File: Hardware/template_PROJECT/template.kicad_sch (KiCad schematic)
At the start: 7 parts

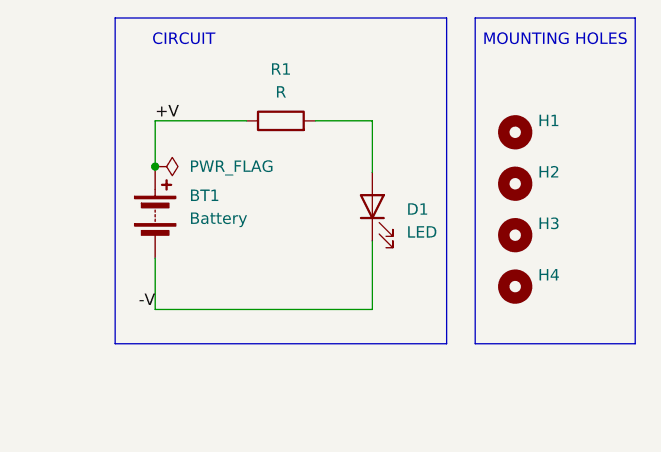
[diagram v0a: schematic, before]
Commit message: creating errors to check
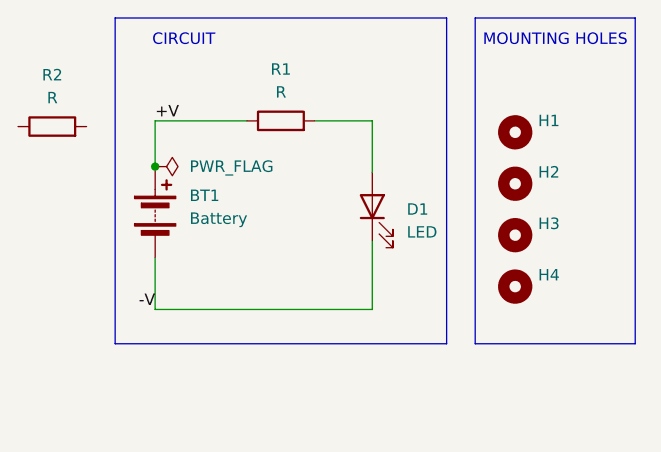
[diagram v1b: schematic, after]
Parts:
- added R2: R, Resistor_SMD:R_0805_2012Metric, symbol Device:R
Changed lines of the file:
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@@
+		)
+	)
+	(symbol
+		(lib_id "Device:R")
+		(at 120.65 92.71 90)
+		(unit 1)
+		(exclude_from_sim no)
+		(in_bom yes)
+		(on_board yes)
+		(dnp no)
+		(fields_autoplaced yes)
+		(property "Reference" "R2"
+			(at 120.65 86.995 90)
+			(effects
+				(font
+					(size 1.27 1.27)
+				)
+			)
+		)
+		(property "Value" "R"
+			(at 120.65 89.535 90)
+			(effects
+				(font
+					(size 1.27 1.27)
+				)
+			)
+		)
+		(property "Footprint" "Resistor_SMD:R_0805_2012Metric"
+			(at 120.65 94.488 90)
+			(effects
+				(font
+					(size 1.27 1.27)
+				)
+				(hide yes)
+			)
+		)
+		(property "Datasheet" "~"
+			(at 120.65 92.71 0)
+			(effects
+				(font
+					(size 1.27 1.27)
+				)
+				(hide yes)
+			)
+		)
+		(property "Description" "Resistor"
+			(at 120.65 92.71 0)
+			(effects
+				(font
+					(size 1.27 1.27)
+				)
+				(hide yes)
+			)
+		)
+		(pin "1"
+		)
+		(pin "2"
+		)
+		(instances
+			(project "template"
+				(path "/92a86815-0425-4ac3-80bb-037195814139"
+					(reference "R2")
+					(unit 1)
+				)
+			)
 		)
 	)

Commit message: worked
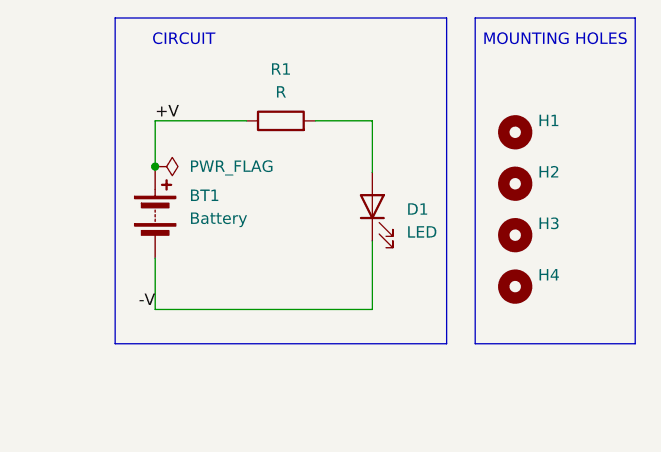
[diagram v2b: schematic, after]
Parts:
- removed R2: R, Resistor_SMD:R_0805_2012Metric, symbol Device:R
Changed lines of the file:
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@@
-		)
-	)
-	(symbol
-		(lib_id "Device:R")
-		(at 120.65 92.71 90)
-		(unit 1)
-		(exclude_from_sim no)
-		(in_bom yes)
-		(on_board yes)
-		(dnp no)
-		(fields_autoplaced yes)
-		(property "Reference" "R2"
-			(at 120.65 86.995 90)
-			(effects
-				(font
-					(size 1.27 1.27)
-				)
-			)
-		)
-		(property "Value" "R"
-			(at 120.65 89.535 90)
-			(effects
-				(font
-					(size 1.27 1.27)
-				)
-			)
-		)
-		(property "Footprint" "Resistor_SMD:R_0805_2012Metric"
-			(at 120.65 94.488 90)
-			(effects
-				(font
-					(size 1.27 1.27)
-				)
-				(hide yes)
-			)
-		)
-		(property "Datasheet" "~"
-			(at 120.65 92.71 0)
-			(effects
-				(font
-					(size 1.27 1.27)
-				)
-				(hide yes)
-			)
-		)
-		(property "Description" "Resistor"
-			(at 120.65 92.71 0)
-			(effects
-				(font
-					(size 1.27 1.27)
-				)
-				(hide yes)
-			)
-		)
-		(pin "1"
-		)
-		(pin "2"
-		)
-		(instances
-			(project "template"
-				(path "/92a86815-0425-4ac3-80bb-037195814139"
-					(reference "R2")
-					(unit 1)
-				)
-			)
 		)
 	)

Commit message: should fail now
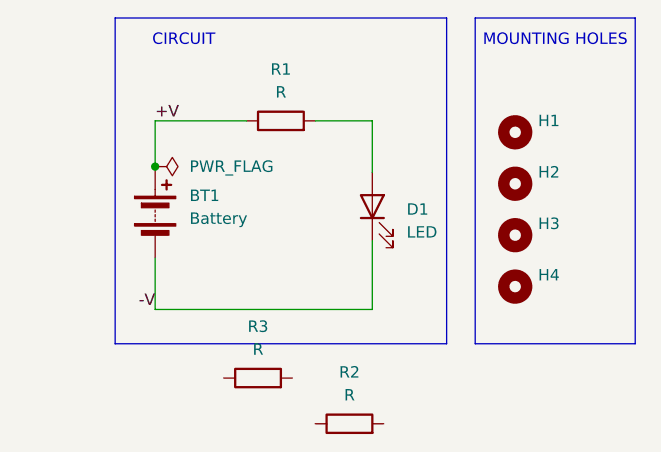
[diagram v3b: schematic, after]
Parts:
- added R2, R3: R, Resistor_SMD:R_0805_2012Metric, symbol Device:R
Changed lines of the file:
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@@
+		)
+	)
+	(symbol
+		(lib_id "Device:R")
+		(at 153.67 125.73 90)
+		(unit 1)
+		(exclude_from_sim no)
+		(in_bom yes)
+		(on_board yes)
+		(dnp no)
+		(fields_autoplaced yes)
+		(property "Reference" "R2"
+			(at 153.67 120.015 90)
+			(effects
+				(font
+					(size 1.27 1.27)
+				)
+			)
+		)
+		(property "Value" "R"
+			(at 153.67 122.555 90)
+			(effects
+				(font
+					(size 1.27 1.27)
+				)
+			)
+		)
+		(property "Footprint" "Resistor_SMD:R_0805_2012Metric"
+			(at 153.67 127.508 90)
+			(effects
+				(font
+					(size 1.27 1.27)
+				)
+				(hide yes)
+			)
+		)
+		(property "Datasheet" "~"
+			(at 153.67 125.73 0)
+			(effects
+				(font
+					(size 1.27 1.27)
+				)
+				(hide yes)
+			)
+		)
+		(property "Description" "Resistor"
+			(at 153.67 125.73 0)
+			(effects
+				(font
+					(size 1.27 1.27)
+				)
+				(hide yes)
+			)
+		)
+		(pin "1"
+		)
+		(pin "2"
+		)
+		(instances
+			(project "template"
+				(path "/92a86815-0425-4ac3-80bb-037195814139"
+					(reference "R2")
+					(unit 1)
+				)
+			)
+		)
+	)
+	(symbol
+		(lib_id "Device:R")
+		(at 143.51 120.65 90)
+		(unit 1)
+		(exclude_from_sim no)
+		(in_bom yes)
+		(on_board yes)
+		(dnp no)
+		(fields_autoplaced yes)
+		(property "Reference" "R3"
+			(at 143.51 114.935 90)
+			(effects
+				(font
+					(size 1.27 1.27)
+				)
+			)
+		)
+		(property "Value" "R"
+			(at 143.51 117.475 90)
+			(effects
+				(font
+					(size 1.27 1.27)
+				)
+			)
+		)
+		(property "Footprint" "Resistor_SMD:R_0805_2012Metric"
+			(at 143.51 122.428 90)
+			(effects
+				(font
+					(size 1.27 1.27)
+				)
+				(hide yes)
+			)
+		)
+		(property "Datasheet" "~"
+			(at 143.51 120.65 0)
+			(effects
+				(font
+					(size 1.27 1.27)
+				)
+				(hide yes)
+			)
+		)
+		(property "Description" "Resistor"
+			(at 143.51 120.65 0)
+			(effects
+				(font
+					(size 1.27 1.27)
+				)
+				(hide yes)
+			)
+		)
+		(pin "1"
+		)
+		(pin "2"
+		)
+		(instances
+			(project "template"
+				(path "/92a86815-0425-4ac3-80bb-037195814139"
+					(reference "R3")
+					(unit 1)
+				)
+			)
 		)
 	)

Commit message: shouldnt fail now
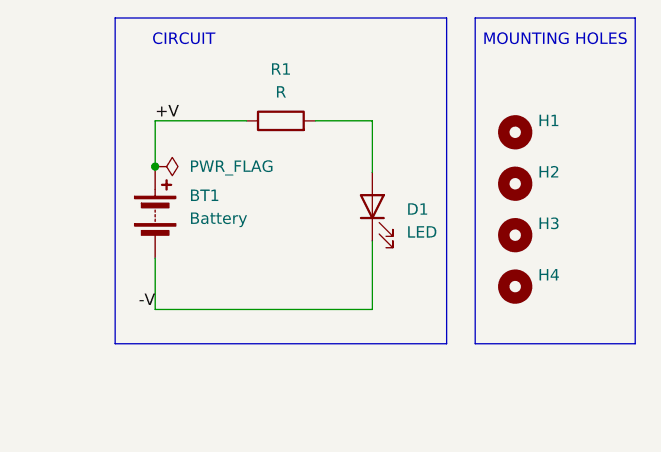
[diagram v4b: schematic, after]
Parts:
- removed R2, R3: R, Resistor_SMD:R_0805_2012Metric, symbol Device:R
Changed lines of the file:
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@@
-		)
-	)
-	(symbol
-		(lib_id "Device:R")
-		(at 153.67 125.73 90)
-		(unit 1)
-		(exclude_from_sim no)
-		(in_bom yes)
-		(on_board yes)
-		(dnp no)
-		(fields_autoplaced yes)
-		(property "Reference" "R2"
-			(at 153.67 120.015 90)
-			(effects
-				(font
-					(size 1.27 1.27)
-				)
-			)
-		)
-		(property "Value" "R"
-			(at 153.67 122.555 90)
-			(effects
-				(font
-					(size 1.27 1.27)
-				)
-			)
-		)
-		(property "Footprint" "Resistor_SMD:R_0805_2012Metric"
-			(at 153.67 127.508 90)
-			(effects
-				(font
-					(size 1.27 1.27)
-				)
-				(hide yes)
-			)
-		)
-		(property "Datasheet" "~"
-			(at 153.67 125.73 0)
-			(effects
-				(font
-					(size 1.27 1.27)
-				)
-				(hide yes)
-			)
-		)
-		(property "Description" "Resistor"
-			(at 153.67 125.73 0)
-			(effects
-				(font
-					(size 1.27 1.27)
-				)
-				(hide yes)
-			)
-		)
-		(pin "1"
-		)
-		(pin "2"
-		)
-		(instances
-			(project "template"
-				(path "/92a86815-0425-4ac3-80bb-037195814139"
-					(reference "R2")
-					(unit 1)
-				)
-			)
-		)
-	)
-	(symbol
-		(lib_id "Device:R")
-		(at 143.51 120.65 90)
-		(unit 1)
-		(exclude_from_sim no)
-		(in_bom yes)
-		(on_board yes)
-		(dnp no)
-		(fields_autoplaced yes)
-		(property "Reference" "R3"
-			(at 143.51 114.935 90)
-			(effects
-				(font
-					(size 1.27 1.27)
-				)
-			)
-		)
-		(property "Value" "R"
-			(at 143.51 117.475 90)
-			(effects
-				(font
-					(size 1.27 1.27)
-				)
-			)
-		)
-		(property "Footprint" "Resistor_SMD:R_0805_2012Metric"
-			(at 143.51 122.428 90)
-			(effects
-				(font
-					(size 1.27 1.27)
-				)
-				(hide yes)
-			)
-		)
-		(property "Datasheet" "~"
-			(at 143.51 120.65 0)
-			(effects
-				(font
-					(size 1.27 1.27)
-				)
-				(hide yes)
-			)
-		)
-		(property "Description" "Resistor"
-			(at 143.51 120.65 0)
-			(effects
-				(font
-					(size 1.27 1.27)
-				)
-				(hide yes)
-			)
-		)
-		(pin "1"
-		)
-		(pin "2"
-		)
-		(instances
-			(project "template"
-				(path "/92a86815-0425-4ac3-80bb-037195814139"
-					(reference "R3")
-					(unit 1)
-				)
-			)
 		)
 	)
